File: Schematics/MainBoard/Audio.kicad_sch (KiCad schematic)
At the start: 13 parts, among them J6 AudioJack3, U11 LM386

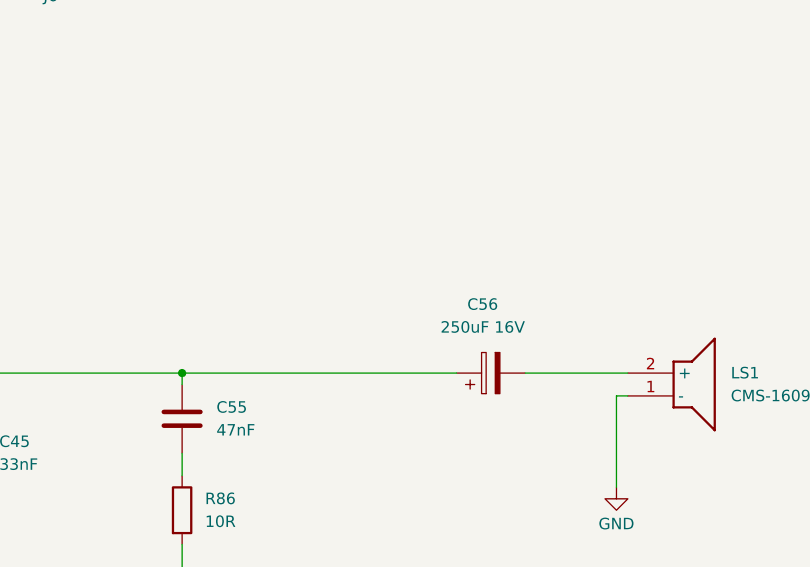
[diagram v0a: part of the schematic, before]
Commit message: Work on PCB
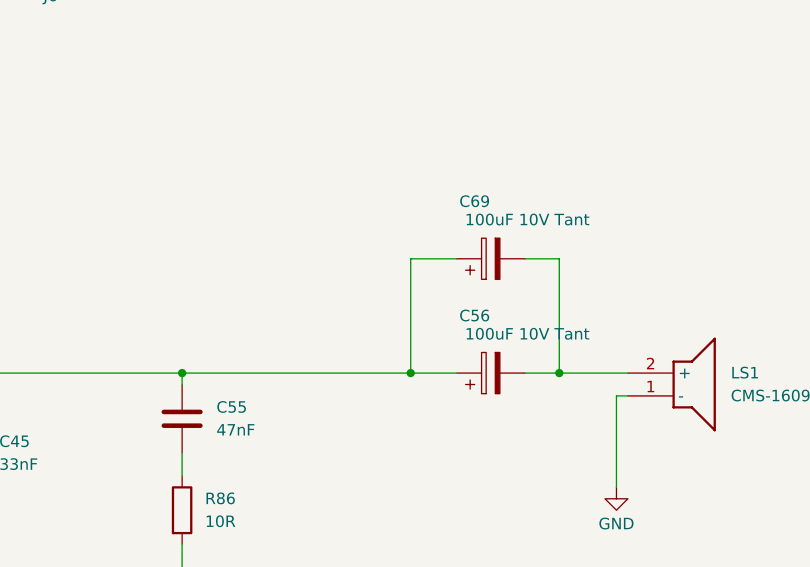
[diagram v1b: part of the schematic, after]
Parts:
- added C69: 100uF 10V Tant, Capacitor_Tantalum_SMD:CP_EIA-7343-30_AVX-N, symbol Device:C_Polarized
- C46, C55: footprint Capacitor_SMD:C_0603_1608Metric -> Capacitor_SMD:C_0402_1005Metric
- C56: value 250uF 16V -> 100uF 10V Tant; footprint Capacitor_SMD:CP_Elec_10x12.5 -> Capacitor_Tantalum_SMD:CP_EIA-7343-30_AVX-N; LCSC DNF -> DNP; Mouser Part Number 667-EEV-FK1V681Q -> (none)
- LS1: footprint CMS160925078SP67 -> CMS-160925-078SP-67:CMS160925078SP67
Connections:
- net at C45.1, C55.1, C56.1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: now also C69.1
- net at C56.2, LS1.2 (+): now also C69.2
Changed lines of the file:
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@@
+	)
+	(junction
+		(at 229.87 92.71)
+		(diameter 0)
+		(color 0 0 0 0)
 	)
 	(junction
@@
 	)
 	(junction
+		(at 213.36 92.71)
+		(diameter 0)
+		(color 0 0 0 0)
+	)
+	(junction
 		(at 81.28 90.17)
 		(diameter 0)
@@
 	(wire
 		(pts
+			(xy 213.36 92.71) (xy 218.44 92.71)
+		)
+		(stroke
+			(width 0)
+			(type default)
+		)
+	)
+	(wire
+		(pts
 			(xy 156.21 107.95) (xy 163.83 107.95)
 		)
@@
 	(wire
 		(pts
+			(xy 226.06 80.01) (xy 229.87 80.01)
+		)
+		(stroke
+			(width 0)
+			(type default)
+		)
+	)
+	(wire
+		(pts
 			(xy 114.3 166.37) (xy 116.84 166.37)
 		)
@@
 	(wire
 		(pts
+			(xy 213.36 80.01) (xy 213.36 92.71)
+		)
+		(stroke
+			(width 0)
+			(type default)
+		)
+	)
+	(wire
+		(pts
 			(xy 128.27 80.01) (xy 134.62 80.01)
 		)
@@
 	(wire
 		(pts
-			(xy 187.96 92.71) (xy 218.44 92.71)
+			(xy 187.96 92.71) (xy 213.36 92.71)
 		)
 		(stroke
@@
 	(wire
 		(pts
+			(xy 218.44 80.01) (xy 213.36 80.01)
+		)
+		(stroke
+			(width 0)
+			(type default)
+		)
+	)
+	(wire
+		(pts
 			(xy 45.72 140.97) (xy 58.42 140.97)
 		)
@@
 	(wire
 		(pts
+			(xy 229.87 80.01) (xy 229.87 92.71)
+		)
+		(stroke
+			(width 0)
+			(type default)
+		)
+	)
+	(wire
+		(pts
 			(xy 81.28 90.17) (xy 129.54 90.17)
 		)
@@
 	(wire
 		(pts
-			(xy 226.06 92.71) (xy 237.49 92.71)
+			(xy 226.06 92.71) (xy 229.87 92.71)
 		)
 		(stroke
@@
 		(pts
 			(xy 187.96 111.76) (xy 187.96 114.3)
+		)
+		(stroke
+			(width 0)
+			(type default)
+		)
+	)
+	(wire
+		(pts
+			(xy 229.87 92.71) (xy 237.49 92.71)
 		)
 		(stroke
@@
 				(path "/a2243a34-697c-4939-97f7-df548e421864/598e71c9-5c06-425f-ac54-aba71004555d"
 					(reference "#PWR0185")
-					(unit 1)
-				)
-			)
-		)
-	)
-	(symbol
-		(lib_id "Device:C_Polarized")
-		(at 222.25 92.71 90)
-		(unit 1)
-		(exclude_from_sim no)
-		(in_bom yes)
-		(on_board yes)
-		(dnp no)
-		(fields_autoplaced yes)
-		(property "Reference" "C56"
-			(at 221.361 85.09 90)
-			(effects
-				(font
-					(size 1.27 1.27)
-				)
-			)
-		)
-		(property "Value" "250uF 16V"
-			(at 221.361 87.63 90)
-			(effects
-				(font
-					(size 1.27 1.27)
-				)
-			)
-		)
-		(property "Footprint" "Capacitor_SMD:CP_Elec_10x12.5"
-			(at 226.06 91.7448 0)
-			(effects
-				(font
-					(size 1.27 1.27)
-				)
-				(hide yes)
-			)
-		)
-		(property "Datasheet" "~"
-			(at 222.25 92.71 0)
-			(effects
-				(font
-					(size 1.27 1.27)
-				)
-				(hide yes)
-			)
-		)
-		(property "Description" "Polarized capacitor"
-			(at 222.25 92.71 0)
-			(effects
-				(font
-					(size 1.27 1.27)
-				)
-				(hide yes)
-			)
-		)
-		(property "Mouser Part Number" "667-EEV-FK1V681Q"
-			(at 222.25 92.71 90)
-			(effects
-				(font
-					(size 1.27 1.27)
-				)
-				(hide yes)
-			)
-		)
-		(property "LCSC" "DNF"
-			(at 222.25 92.71 90)
-			(effects
-				(font
-					(size 1.27 1.27)
-				)
-				(hide yes)
-			)
-		)
-		(pin "1"
-		)
-		(pin "2"
-		)
-		(instances
-			(project ""
-				(path "/a2243a34-697c-4939-97f7-df548e421864/598e71c9-5c06-425f-ac54-aba71004555d"
-					(reference "C56")
 					(unit 1)
 				)
@@
 	)
 	(symbol
+		(lib_id "Device:C_Polarized")
+		(at 222.25 80.01 90)
+		(unit 1)
+		(exclude_from_sim no)
+		(in_bom yes)
+		(on_board yes)
+		(dnp no)
+		(property "Reference" "C69"
+			(at 220.472 73.66 90)
+			(effects
+				(font
+					(size 1.27 1.27)
+				)
+			)
+		)
+		(property "Value" "100uF 10V Tant"
+			(at 226.314 75.692 90)
+			(effects
+				(font
+					(size 1.27 1.27)
+				)
+			)
+		)
+		(property "Footprint" "Capacitor_Tantalum_SMD:CP_EIA-7343-30_AVX-N"
+			(at 226.06 79.0448 0)
+			(effects
+				(font
+					(size 1.27 1.27)
+				)
+				(hide yes)
+			)
+		)
+		(property "Datasheet" "~"
+			(at 222.25 80.01 0)
+			(effects
+				(font
+					(size 1.27 1.27)
+				)
+				(hide yes)
+			)
+		)
+		(property "Description" "Polarized capacitor"
+			(at 222.25 80.01 0)
+			(effects
+				(font
+					(size 1.27 1.27)
+				)
+				(hide yes)
+			)
+		)
+		(property "LCSC" "DNP"
+			(at 222.25 80.01 0)
+			(effects
+				(font
+					(size 1.27 1.27)
+				)
+				(hide yes)
+			)
+		)
+		(pin "1"
+		)
+		(pin "2"
+		)
+		(instances
+			(project "MainBoard"
+				(path "/a2243a34-697c-4939-97f7-df548e421864/598e71c9-5c06-425f-ac54-aba71004555d"
+					(reference "C69")
+					(unit 1)
+				)
+			)
+		)
+	)
+	(symbol
 		(lib_id "power:GND")
 		(at 121.92 102.87 0)
@@
 			)
 		)
-		(property "Footprint" "CMS160925078SP67"
+		(property "Footprint" "CMS-160925-078SP-67:CMS160925078SP67"
 			(at 248.92 195.25 0)
 			(effects
@@
 			)
 		)
-		(property "Footprint" "Capacitor_SMD:C_0603_1608Metric"
+		(property "Footprint" "Capacitor_SMD:C_0402_1005Metric"
 			(at 128.27 79.0448 0)
 			(effects
@@
 				(path "/a2243a34-697c-4939-97f7-df548e421864/598e71c9-5c06-425f-ac54-aba71004555d"
 					(reference "C46")
+					(unit 1)
+				)
+			)
+		)
+	)
+	(symbol
+		(lib_id "Device:C_Polarized")
+		(at 222.25 92.71 90)
+		(unit 1)
+		(exclude_from_sim no)
+		(in_bom yes)
+		(on_board yes)
+		(dnp no)
+		(property "Reference" "C56"
+			(at 220.472 86.36 90)
+			(effects
+				(font
+					(size 1.27 1.27)
+				)
+			)
+		)
+		(property "Value" "100uF 10V Tant"
+			(at 226.314 88.392 90)
+			(effects
+				(font
+					(size 1.27 1.27)
+				)
+			)
+		)
+		(property "Footprint" "Capacitor_Tantalum_SMD:CP_EIA-7343-30_AVX-N"
+			(at 226.06 91.7448 0)
+			(effects
+				(font
+					(size 1.27 1.27)
+				)
+				(hide yes)
+			)
+		)
+		(property "Datasheet" "~"
+			(at 222.25 92.71 0)
+			(effects
+				(font
+					(size 1.27 1.27)
+				)
+				(hide yes)
+			)
+		)
+		(property "Description" "Polarized capacitor"
+			(at 222.25 92.71 0)
+			(effects
+				(font
+					(size 1.27 1.27)
+				)
+				(hide yes)
+			)
+		)
+		(property "LCSC" "DNP"
+			(at 222.25 92.71 0)
+			(effects
+				(font
+					(size 1.27 1.27)
+				)
+				(hide yes)
+			)
+		)
+		(pin "1"
+		)
+		(pin "2"
+		)
+		(instances
+			(project "MainBoard"
+				(path "/a2243a34-697c-4939-97f7-df548e421864/598e71c9-5c06-425f-ac54-aba71004555d"
+					(reference "C56")
 					(unit 1)
 				)
@@
 			)
 		)
-		(property "Footprint" "Capacitor_SMD:C_0603_1608Metric"
+		(property "Footprint" "Capacitor_SMD:C_0402_1005Metric"
 			(at 188.9252 101.6 0)
 			(effects
